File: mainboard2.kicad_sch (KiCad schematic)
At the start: 47 parts, among them J10 Conn_01x03_Socket, J11 Conn_01x02_Socket, J12 GPIO, J13 Conn_01x02_Socket, J14 Conn_01x03_Socket, J15 Conn_01x03_Socket, J16 Conn_01x03_Socket, J17 Conn_01x03_Socket, J18 Conn_01x03_Socket, J19 Conn_01x03_Socket, J2 Conn_01x02_Socket, J20 Conn_01x04_Socket, J9 Conn_01x03_Socket, Q5 IRFML8244TRPBF, U4 MCP3208, U5 PCA9685PW, U7 PCA9685PW

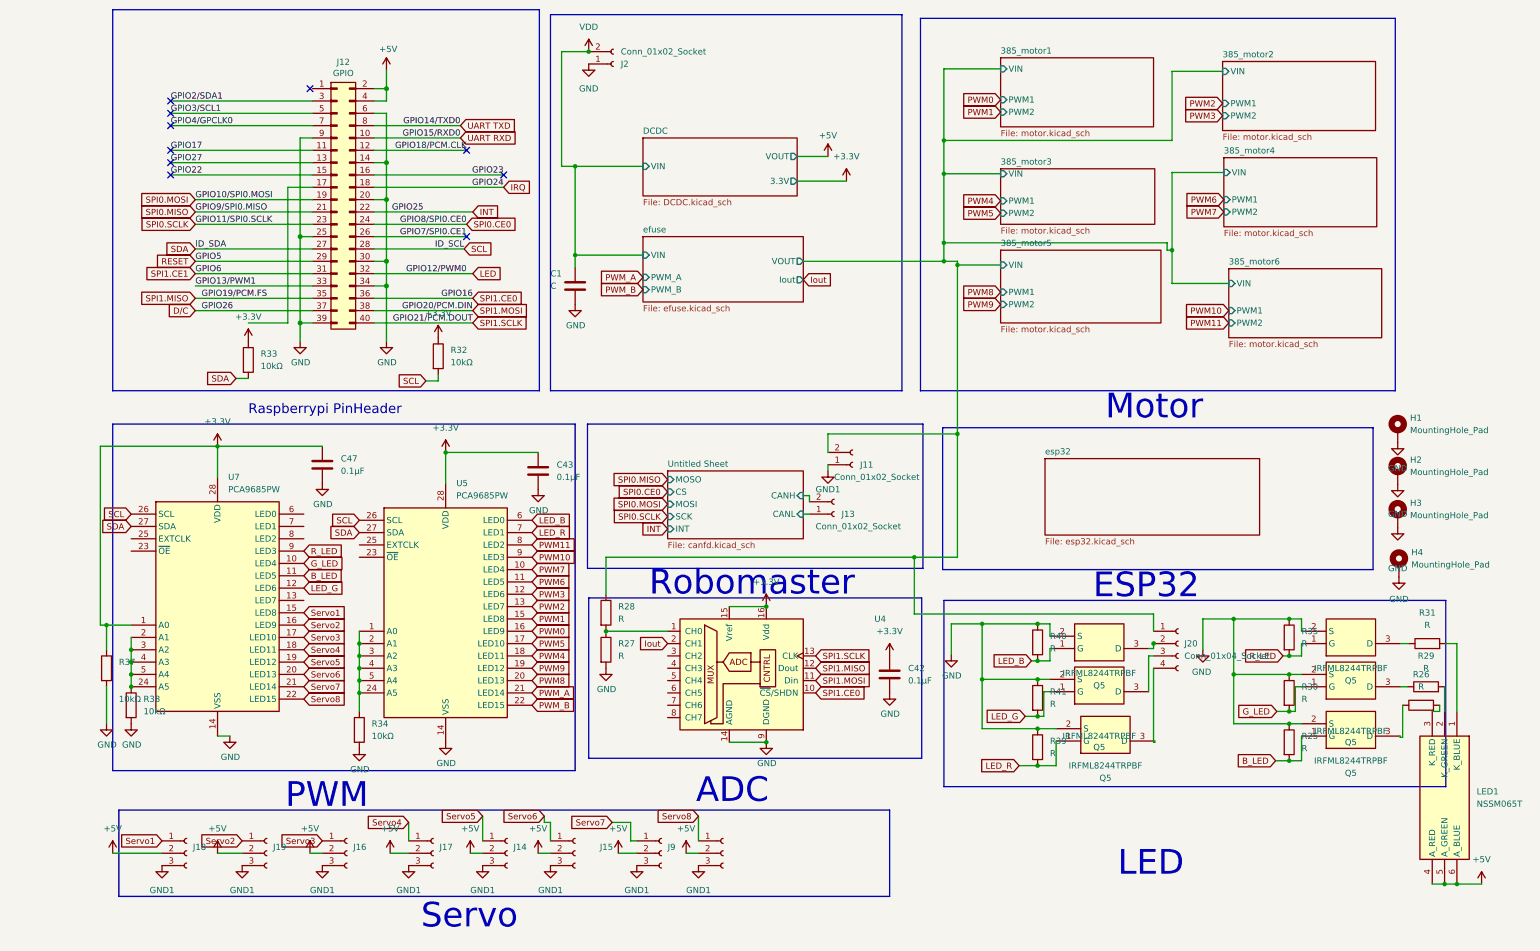
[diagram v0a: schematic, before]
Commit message: ESP32バージョン
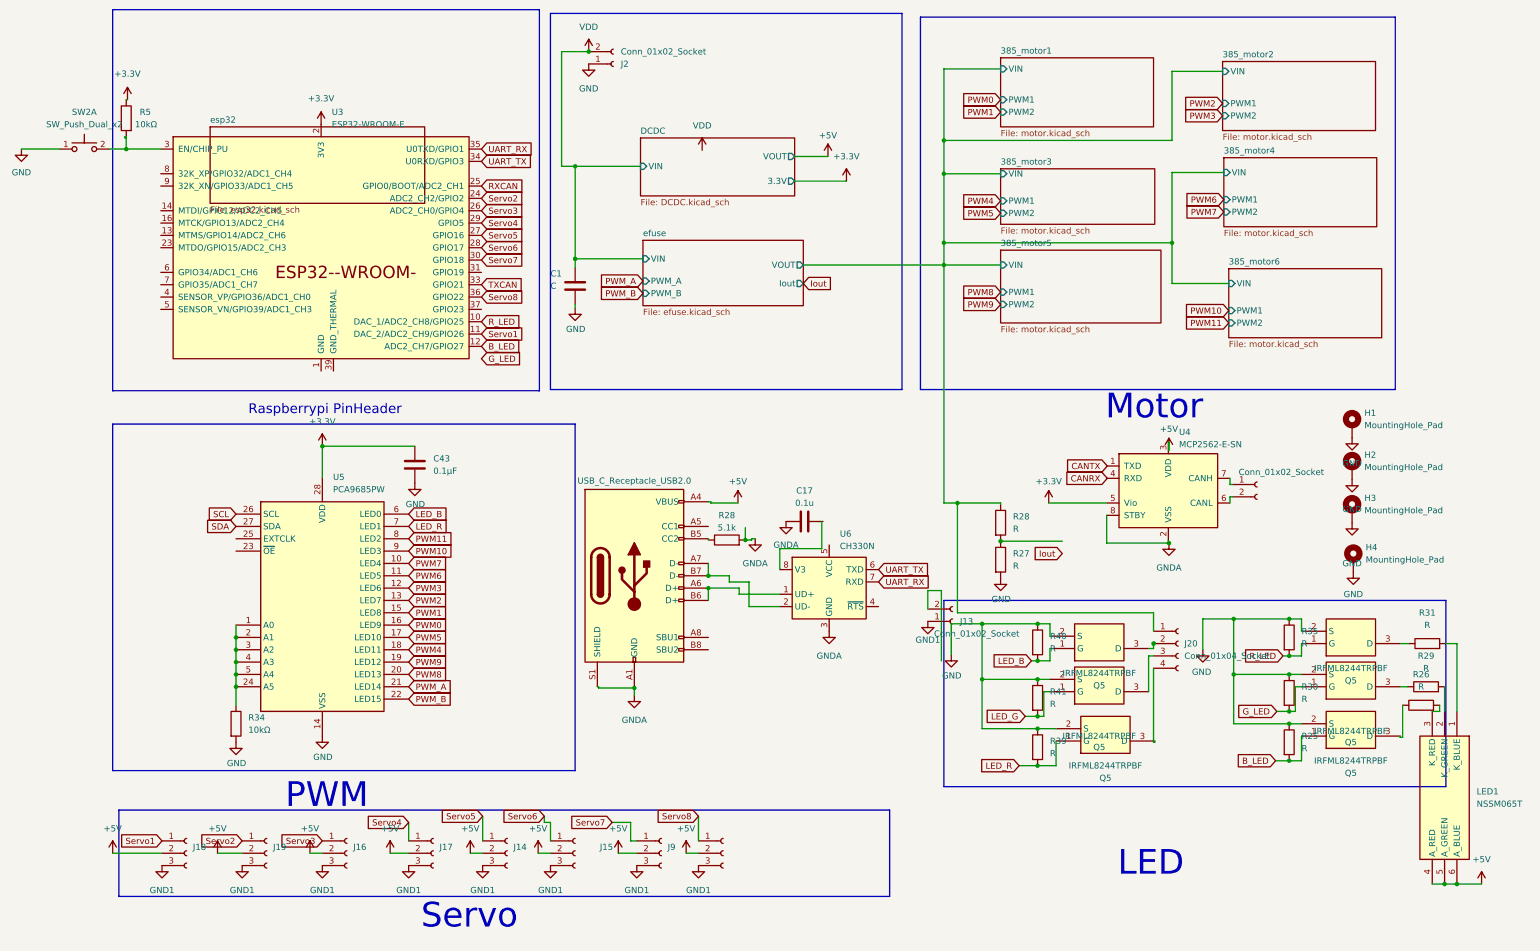
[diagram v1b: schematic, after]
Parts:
- removed C42, C47: 0.1μF, Capacitor_SMD:C_0603_1608Metric_Pad1.08x0.95mm_HandSolder, symbol Device:C
- removed J11: Conn_01x02_Socket, Connector_AMASS:AMASS_XT30PW-M_1x02_P2.50mm_Horizontal, symbol Connector:Conn_01x02_Socket
- removed J12: GPIO, Connector_PinSocket_2.54mm:PinSocket_2x20_P2.54mm_Vertical, symbol Connector_Generic:Conn_02x20_Odd_Even
- removed R32, R33, R37, R38: 10kΩ, Resistor_SMD:R_0603_1608Metric_Pad0.98x0.95mm_HandSolder, symbol Device:R
- removed U4: MCP3208, Library:SOIC127P600X175-16N, symbol Analog_ADC:MCP3208
- removed U7: PCA9685PW, Package_SO:TSSOP-28_4.4x9.7mm_P0.65mm, symbol Driver_LED:PCA9685PW
- added C17: 0.1u, Capacitor_SMD:C_0603_1608Metric_Pad1.08x0.95mm_HandSolder, symbol Device:C
- added J12: Conn_01x02_Socket, Connector_JST:JST_XH_B2B-XH-A_1x02_P2.50mm_Vertical, symbol Connector:Conn_01x02_Socket
- added J13: USB_C_Receptacle_USB2.0, Connector_USB:USB_C_Receptacle_HCTL_HC-TYPE-C-16P-01A, symbol Connector:USB_C_Receptacle_USB2.0
- added R28: 5.1k, Resistor_SMD:R_0603_1608Metric_Pad0.98x0.95mm_HandSolder, symbol Device:R
- added R5: 10kΩ, Resistor_SMD:R_0603_1608Metric_Pad0.98x0.95mm_HandSolder, symbol Device:R
- added SW2: SW_Push_Dual_x2, Button_Switch_SMD:SW_Push_1P1T_NO_CK_KMR2, symbol Switch:SW_Push_Dual_x2
- added U3: ESP32-WROOM-E, PCM_Espressif:ESP32-WROOM-32E, symbol PCM_Espressif:ESP32-WROOM-E
- added U4: MCP2562-E-SN, Package_SO:SOIC-8_3.9x4.9mm_P1.27mm, symbol Interface_CAN_LIN:MCP2562-E-SN
- added U6: CH330N, Package_SO:SOIC-8_3.9x4.9mm_P1.27mm, symbol Interface_USB:CH330N
- J13: footprint Connector_JST:JST_XH_B2B-XH-A_1x02_P2.50mm_Vertical -> Connector_AMASS:AMASS_XT30PW-F_1x02_P2.50mm_Horizontal
- J20: footprint Connector_JST:JST_XH_S4B-XH-A_1x04_P2.50mm_Horizontal -> Connector_JST:JST_XH_B4B-XH-A_1x04_P2.50mm_Vertical
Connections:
- net Untitled Sheet/CANL is gone; now on net GND1: J13.1 (Pin_1)
- net +3.3V: now also R5.1, U3.2 (3V3), U4.5 (Vio)
- net +5V: now also J13.A4 (VBUS), J13.A9 (VBUS), J13.B4 (VBUS), J13.B9 (VBUS), U4.3 (VDD)
- net B_LED: now also U3.12 (ADC2_CH7/GPIO27)
- net GND: now also SW2.1 (C)
- net R_LED: now also U3.10 (DAC_1/ADC2_CH8/GPIO25)
- net Servo1: now also U3.11 (DAC_2/ADC2_CH9/GPIO26)
- net Servo2: now also U3.24 (ADC2_CH2/GPIO2)
- net Servo3: now also U3.26 (ADC2_CH0/GPIO4)
- net Servo4: now also U3.29 (GPIO5)
- net Servo5: now also U3.27 (GPIO16)
- net Servo6: now also U3.28 (GPIO17)
- net Servo7: now also U3.30 (GPIO18)
- net Servo8: now also U3.36 (GPIO22)
- net Untitled Sheet/CANH: no longer names the net of J13.2 (Pin_2)
- new net: U3.1 (GND), U3.15 (GND), U3.38 (GND)
- new net: R5.2, SW2.2 (D), U3.3 (EN/CHIP_PU)
- new net: J13.B5 (CC2), R28.1
- new net: J12.2 (Pin_2), U4.6 (CANL)
- new net: J12.1 (Pin_1), U4.7 (CANH)
- new net: J13.A6 (D+), J13.B6 (D+), U6.1 (UD+)
- new net: J13.A7 (D-), J13.B7 (D-), U6.2 (UD-)
- new net CANRX: U4.4 (RXD)
- new net CANTX: U4.1 (TXD)
- new net GNDA: C17.1, J13.A1 (GND), J13.A12 (GND), J13.B1 (GND), J13.B12 (GND), J13.S1 (SHIELD), R28.2, U4.2 (VSS), U4.8 (STBY), U6.3 (GND)
- new net RXCAN: U3.25 (GPIO0/BOOT/ADC2_CH1)
- new net TXCAN: U3.33 (GPIO21)
- new net UART_RX: U3.35 (U0TXD/GPIO1), U6.7 (RXD)
- new net UART_TX: U3.34 (U0RXD/GPIO3), U6.6 (TXD)
- no-connect marks 10 -> 0
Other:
- removed sheet Untitled Sheet
- note removed: "ADC"
- note removed: "ESP32"
- note removed: "Robomaster"
- moved on the sheet: C43, H1, H2, H3, H4, R27, R28, R34, U5
